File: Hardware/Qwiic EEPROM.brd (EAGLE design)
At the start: 25.4 x 25.4 mm, 60 parts, among them J2 QWIIC_RA, J4 QWIIC_RA, U1 RM24C512C

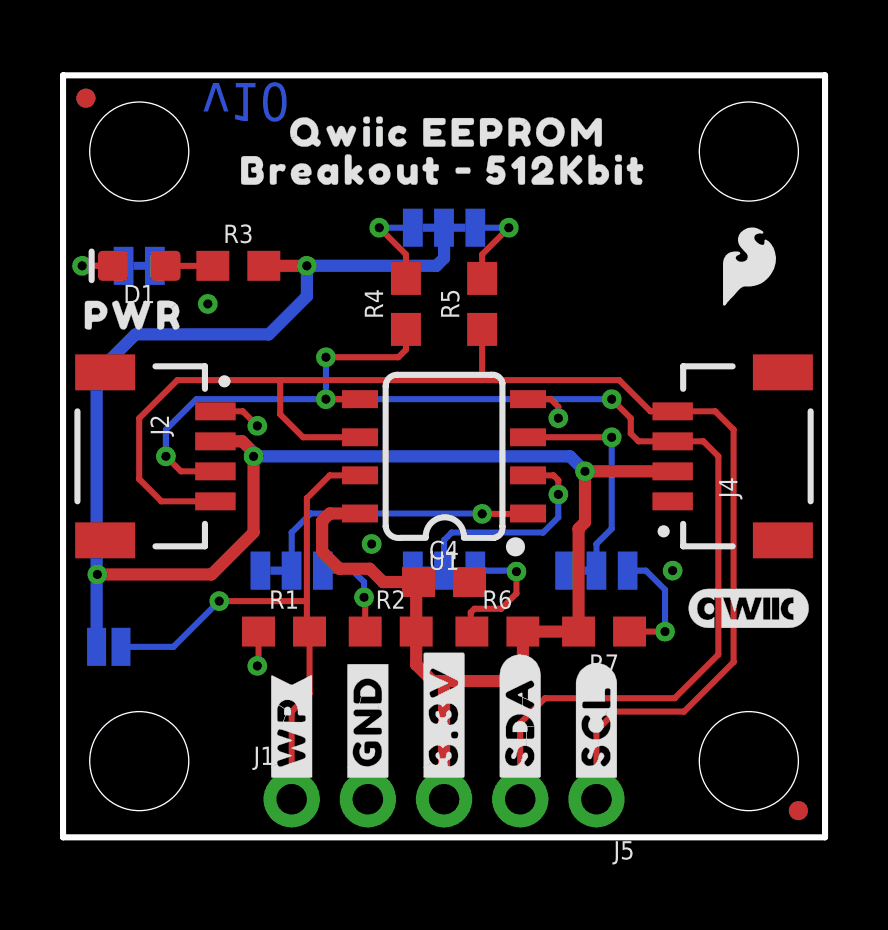
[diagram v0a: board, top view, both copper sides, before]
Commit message: Update Qwiic EEPROM.brd
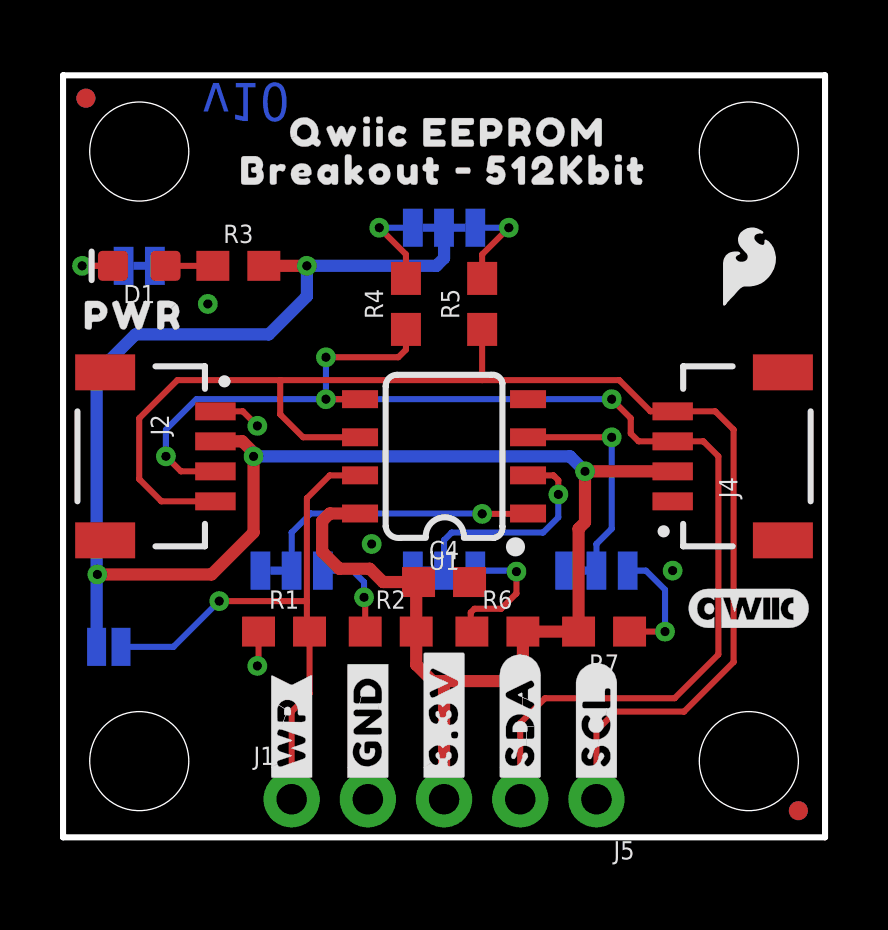
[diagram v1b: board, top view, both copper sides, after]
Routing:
- net GND: track 4.25 -> 2.76 mm, vias 6 -> 5
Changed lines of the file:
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@@
 <layer number="39" name="tKeepout" color="4" fill="11" visible="no" active="yes"/>
 <layer number="40" name="bKeepout" color="1" fill="11" visible="no" active="yes"/>
-<layer number="41" name="tRestrict" color="4" fill="10" visible="no" active="yes"/>
+<layer number="41" name="tRestrict" color="4" fill="10" visible="yes" active="yes"/>
 <layer number="42" name="bRestrict" color="1" fill="10" visible="no" active="yes"/>
 <layer number="43" name="vRestrict" color="2" fill="10" visible="no" active="yes"/>
@@
 <layer number="45" name="Holes" color="7" fill="1" visible="yes" active="yes"/>
 <layer number="46" name="Milling" color="3" fill="1" visible="no" active="yes"/>
-<layer number="47" name="Measures" color="7" fill="1" visible="no" active="yes"/>
+<layer number="47" name="Measures" color="7" fill="1" visible="yes" active="yes"/>
 <layer number="48" name="Document" color="7" fill="1" visible="no" active="yes"/>
 <layer number="49" name="Reference" color="7" fill="1" visible="no" active="yes"/>
@@
 <wire x1="25.4" y1="0" x2="0" y2="0" width="0.2032" layer="20"/>
 <text x="6.096" y="24.511" size="1.27" layer="16" font="vector" ratio="15" rot="SMR180" align="center">v10</text>
-<rectangle x1="14.351" y1="13.97" x2="14.732" y2="14.986" layer="41"/>
 <text x="17.78" y="-12.7" size="1.778" layer="51" font="vector">Ciara Jekel</text>
 <dimension x1="0" y1="25.4" x2="25.4" y2="25.4" x3="12.7" y3="30.48" textsize="1.778" layer="47" unit="inch"/>
@@
 <via x="6.477" y="13.716" extent="1-16" drill="0.3048"/>
 <via x="6.477" y="5.715" extent="1-16" drill="0.3048"/>
-<via x="16.51" y="13.97" extent="1-16" drill="0.3048"/>
-<wire x1="15.5" y1="14.605" x2="16.256" y2="14.605" width="0.2032" layer="1"/>
-<wire x1="16.51" y1="13.97" x2="16.51" y2="14.351" width="0.2032" layer="1"/>
-<wire x1="16.51" y1="14.351" x2="16.256" y2="14.605" width="0.2032" layer="1"/>
 <wire x1="6.516" y1="6.858" x2="6.516" y2="5.754" width="0.2032" layer="1"/>
 <wire x1="6.516" y1="5.754" x2="6.477" y2="5.715" width="0.2032" layer="1"/>
